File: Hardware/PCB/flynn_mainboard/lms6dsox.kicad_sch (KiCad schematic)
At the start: 5 parts, among them U4 LSM6DSOX

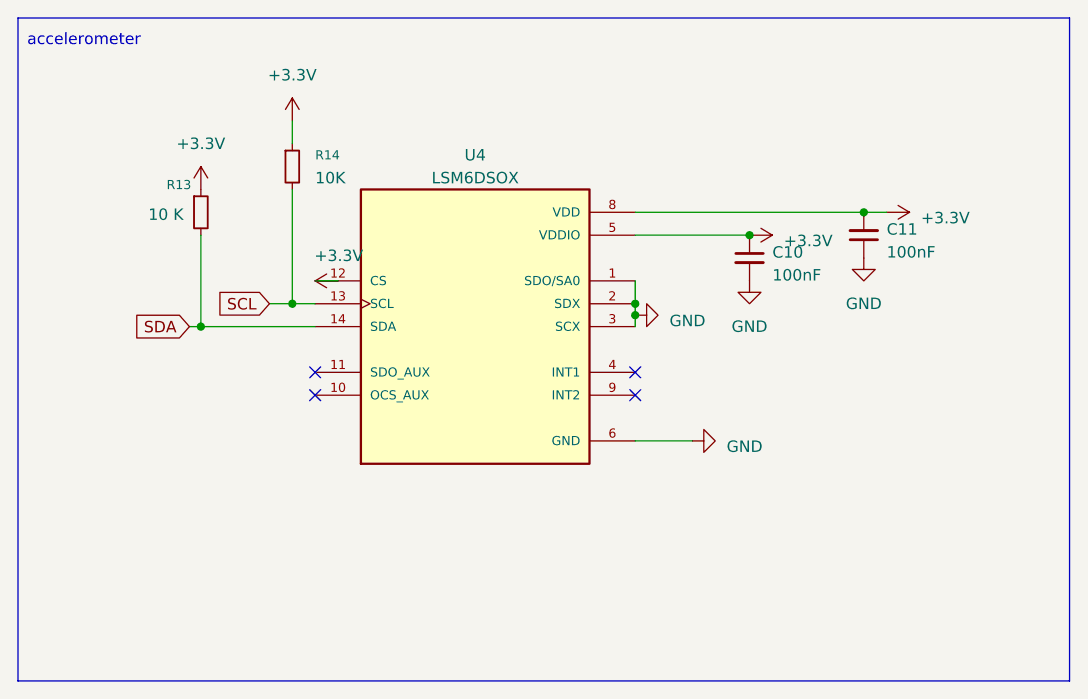
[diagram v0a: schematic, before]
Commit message: Journaling Update
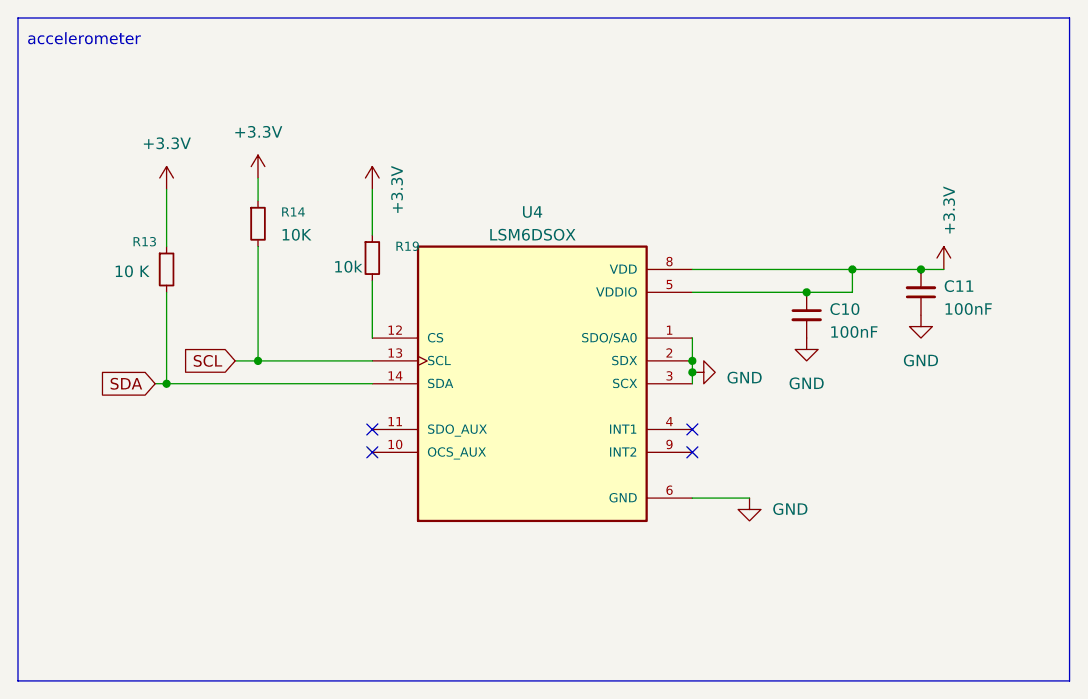
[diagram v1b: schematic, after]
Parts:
- added R19: 10k, Resistor_SMD:R_0603_1608Metric, symbol Device:R_Small
- C10, C11: footprint (none) -> Capacitor_SMD:C_0603_1608Metric
- R13, R14: footprint (none) -> Resistor_SMD:R_0603_1608Metric
- U4: footprint LSM6DSOX:PQFN50P250X300X86-14N -> Package_LGA:LGA-14_3x2.5mm_P0.5mm_LayoutBorder3x4y
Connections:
- net +3.3V: now also R19.1; no longer U4.12 (CS)
- new net: R19.2, U4.12 (CS)
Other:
- moved on the sheet: C10, C11, R13, R14, U4
